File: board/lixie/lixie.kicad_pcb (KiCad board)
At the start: 2 copper layers, 67.5 x 37.8 mm, 43 parts, among them P1 USB_OTG, U1 IS31FL3738, U2 MIC550x, U3 MAX40200, U4 STM32L073xZ

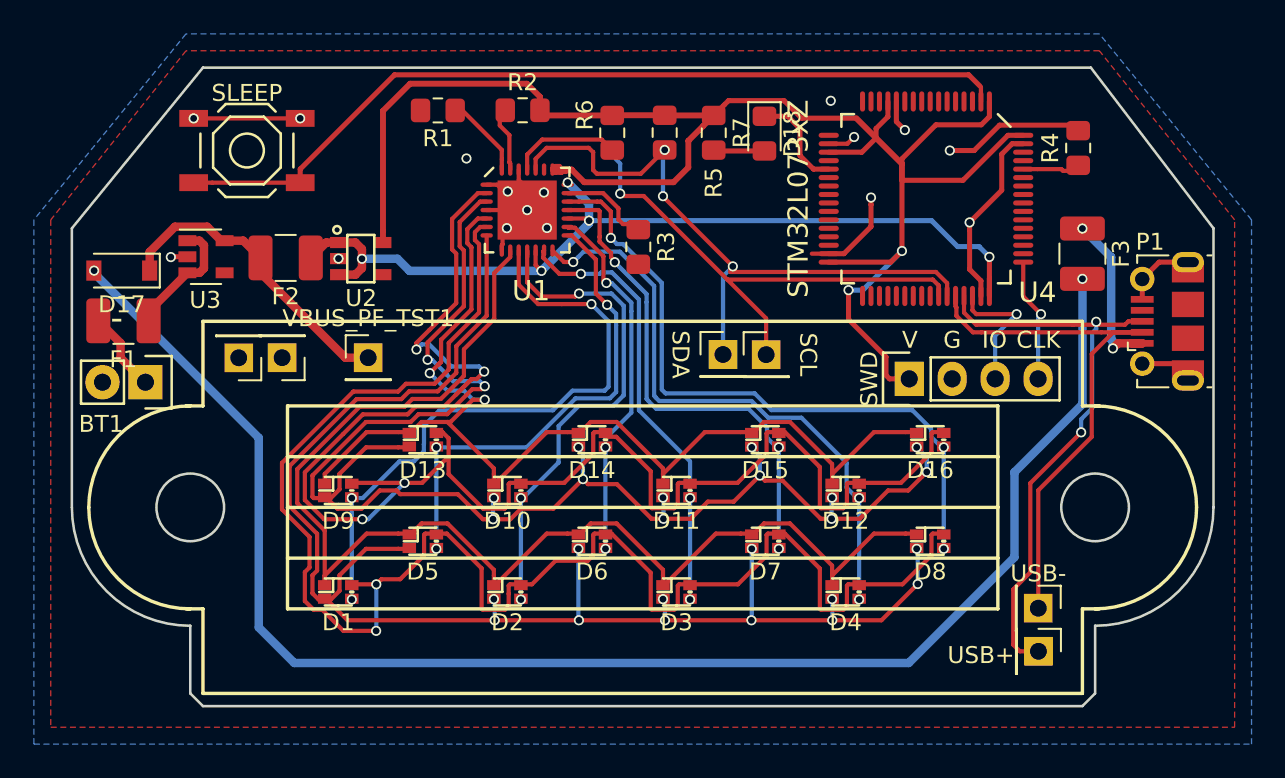
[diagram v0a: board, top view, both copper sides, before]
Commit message: kicad crashed so now I am wiring the LEDs for a fucking 3rd time
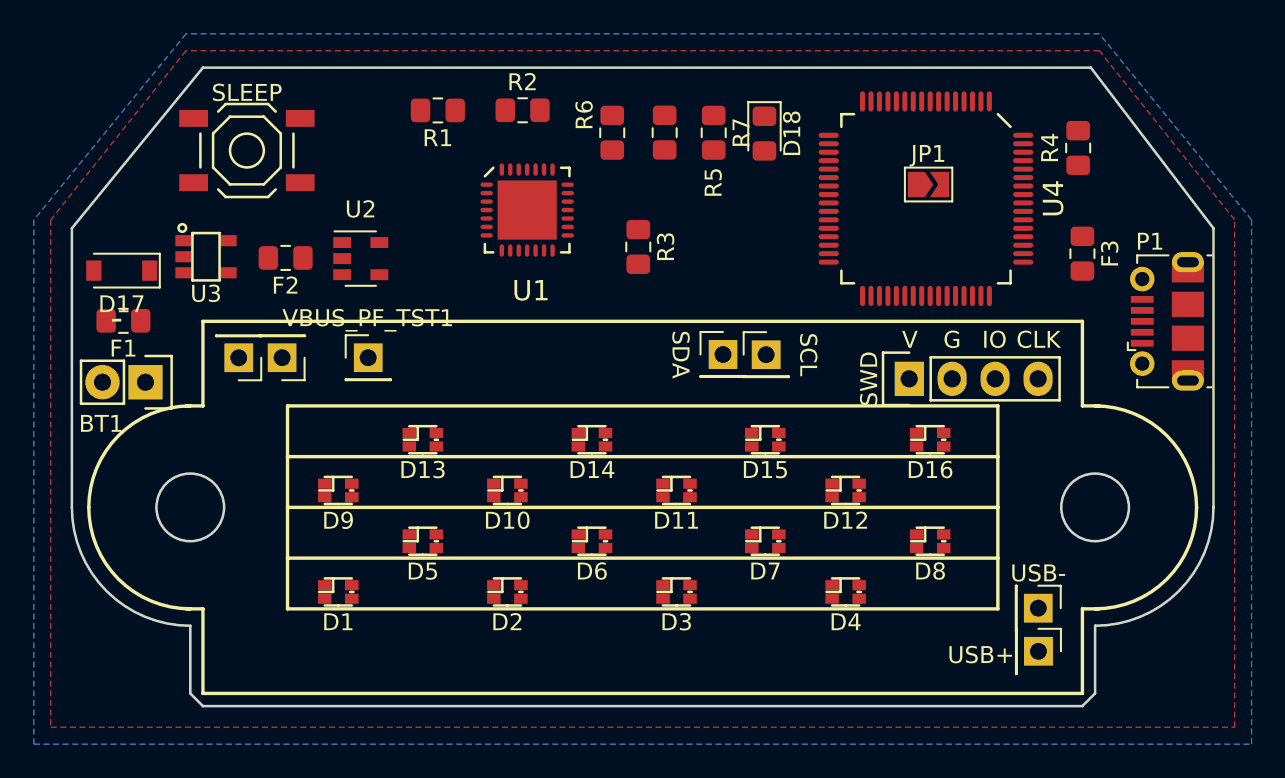
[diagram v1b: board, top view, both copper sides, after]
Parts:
- added JP1: Jumper_2_Open, Jumper:SolderJumper-2_P1.3mm_Open_TrianglePad1.0x1.5mm, F.Cu at (120.9, 68.9)
- D1, D10, D11, D12, D13, D14, D15, D16, D2, D3, D4, D5, D6, D7, D8, D9: value LED_RGAB -> LED_ARBG; footprint lixie:LED_RGAB_0606 -> lixie:LED_LSTD_0606
- F1, F2, F3: footprint Fuse:Fuse_1210_3225Metric_Pad1.42x2.65mm_HandSolder -> Fuse:Fuse_0805_2012Metric_Pad1.15x1.40mm_HandSolder
- R1, R2: value 100k -> 4.7k
- R4: value 10k -> 100k
- R5: value 4.7k -> 100k
- R6: value 4.7k -> R
- R7: value R -> 10k
- U2: value MIC550x -> MAX40200; footprint lixie:MIC550x -> lixie:MAX40200
- U3: value MAX40200 -> MIC550x; footprint lixie:MAX40200 -> lixie:MIC550x
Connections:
- D11 pad 1: Net-(D10-Pad1) -> Net-(D11-Pad1)
- D11 pad 3: Net-(D11-Pad3) -> Net-(D10-Pad3)
- D12 pad 1: Net-(D10-Pad1) -> Net-(D12-Pad1)
- D12 pad 3: Net-(D12-Pad3) -> Net-(D10-Pad3)
- D13 pad 1: Net-(D10-Pad1) -> Net-(D13-Pad1)
- D13 pad 3: Net-(D13-Pad3) -> Net-(D10-Pad3)
- D14 pad 1: Net-(D10-Pad1) -> Net-(D14-Pad1)
- D14 pad 3: Net-(D14-Pad3) -> Net-(D10-Pad3)
- D15 pad 1: Net-(D10-Pad1) -> Net-(D15-Pad1)
- D15 pad 3: Net-(D15-Pad3) -> Net-(D10-Pad3)
- D16 pad 1: Net-(D10-Pad1) -> Net-(D16-Pad1)
- D16 pad 3: Net-(D16-Pad3) -> Net-(D10-Pad3)
- D2 pad 1: Net-(D1-Pad1) -> Net-(D10-Pad1)
- D2 pad 3: Net-(D10-Pad3) -> Net-(D1-Pad3)
- D3 pad 1: Net-(D1-Pad1) -> Net-(D11-Pad1)
- D3 pad 3: Net-(D11-Pad3) -> Net-(D1-Pad3)
- D4 pad 1: Net-(D1-Pad1) -> Net-(D12-Pad1)
- D4 pad 3: Net-(D12-Pad3) -> Net-(D1-Pad3)
- D5 pad 1: Net-(D1-Pad1) -> Net-(D13-Pad1)
- D5 pad 3: Net-(D13-Pad3) -> Net-(D1-Pad3)
- D6 pad 1: Net-(D1-Pad1) -> Net-(D14-Pad1)
- D6 pad 3: Net-(D14-Pad3) -> Net-(D1-Pad3)
- D7 pad 1: Net-(D1-Pad1) -> Net-(D15-Pad1)
- D7 pad 3: Net-(D15-Pad3) -> Net-(D1-Pad3)
- D8 pad 1: Net-(D1-Pad1) -> Net-(D16-Pad1)
- D8 pad 3: Net-(D16-Pad3) -> Net-(D1-Pad3)
- D9 pad 1: Net-(D10-Pad1) -> Net-(D1-Pad1)
- D9 pad 3: Net-(D1-Pad3) -> Net-(D10-Pad3)
- R1 pad 1: /SDB -> +3V3
- R1 pad 2: GND -> /SDA
- R2 pad 1: /INTB -> +3V3
- R2 pad 2: +3V3 -> /SCL
- R3 pad 1: /LED_CURRENT -> /SDB
- R4 pad 1: /BOOT0 -> /INTB
- R4 pad 2: GND -> +3V3
- R5 pad 1: +3V3 -> /LED_CURRENT
- R5 pad 2: /SDA -> GND
- R6 pad 2: /SCL -> Net-(D18-Pad2)
- R7 pad 1: +3V3 -> /BOOT0
- R7 pad 2: Net-(D18-Pad2) -> GND
- U1 pad 10: Net-(D1-Pad3) -> Net-(D1-Pad1)
- U1 pad 11: Net-(D10-Pad3) -> Net-(D10-Pad1)
- U1 pad 13: Net-(D11-Pad3) -> Net-(D11-Pad1)
- U1 pad 14: Net-(D12-Pad3) -> Net-(D12-Pad1)
- U1 pad 15: Net-(D13-Pad3) -> Net-(D13-Pad1)
- U1 pad 16: Net-(D14-Pad3) -> Net-(D14-Pad1)
- U1 pad 18: Net-(D15-Pad3) -> Net-(D15-Pad1)
- U1 pad 19: Net-(D16-Pad3) -> Net-(D16-Pad1)
- U1 pad 2: Net-(D10-Pad4) -> Net-(D10-Pad3)
- U1 pad 3: Net-(D10-Pad2) -> Net-(D10-Pad4)
- U1 pad 5: Net-(D10-Pad1) -> Net-(D10-Pad2)
- U1 pad 6: Net-(D1-Pad4) -> Net-(D1-Pad3)
- U1 pad 7: Net-(D1-Pad2) -> Net-(D1-Pad4)
- U1 pad 9: Net-(D1-Pad1) -> Net-(D1-Pad2)
- U2 pad 1: VBUS -> Net-(F1-Pad1)
- U2 pad 3: VBUS -> Net-(F1-Pad1)
- U2 pad 5: +3V3 -> Net-(D17-Pad1)
- U3 pad 1: Net-(F1-Pad1) -> VBUS
- U3 pad 3: Net-(F1-Pad1) -> VBUS
- U3 pad 5: Net-(D17-Pad1) -> +3V3
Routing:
- net +3V3: track 99.2 -> 0.00 mm, vias 2 -> 0
- net Net-(D10-Pad4): track 95.3 -> 0.00 mm, vias 4 -> 0
- net Net-(D1-Pad4): track 95.0 -> 0.00 mm, vias 2 -> 0
- net Net-(D17-Pad2): track 91.4 -> 0.00 mm, vias 2 -> 0
- net Net-(D10-Pad2): track 88.0 -> 0.00 mm, vias 14 -> 0
- net Net-(D1-Pad2): track 87.8 -> 0.00 mm, vias 12 -> 0
- net Net-(D1-Pad1): track 75.4 -> 0.00 mm
- net Net-(D10-Pad1): track 64.7 -> 0.00 mm, vias 2 -> 0
- net GND: track 54.9 -> 0.00 mm, vias 16 -> 0
- net VBUS: track 54.8 -> 0.00 mm, vias 5 -> 0
- net Net-(SW1-Pad2): track 50.8 -> 0.00 mm
- net Net-(D16-Pad3): track 39.1 -> 0.00 mm, vias 3 -> 0
- net /SDA: track 38.7 -> 0.00 mm, vias 3 -> 0
- net Net-(D1-Pad3): track 36.9 -> 0.00 mm, vias 3 -> 0
- net /SCL: track 36.4 -> 0.00 mm, vias 1 -> 0
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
